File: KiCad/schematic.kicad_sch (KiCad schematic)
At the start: 10 parts, among them J1 AudioJack3, J2 Barrel_Jack_Switch, J3 AudioJack3, SW1 SW_DPDT_x2

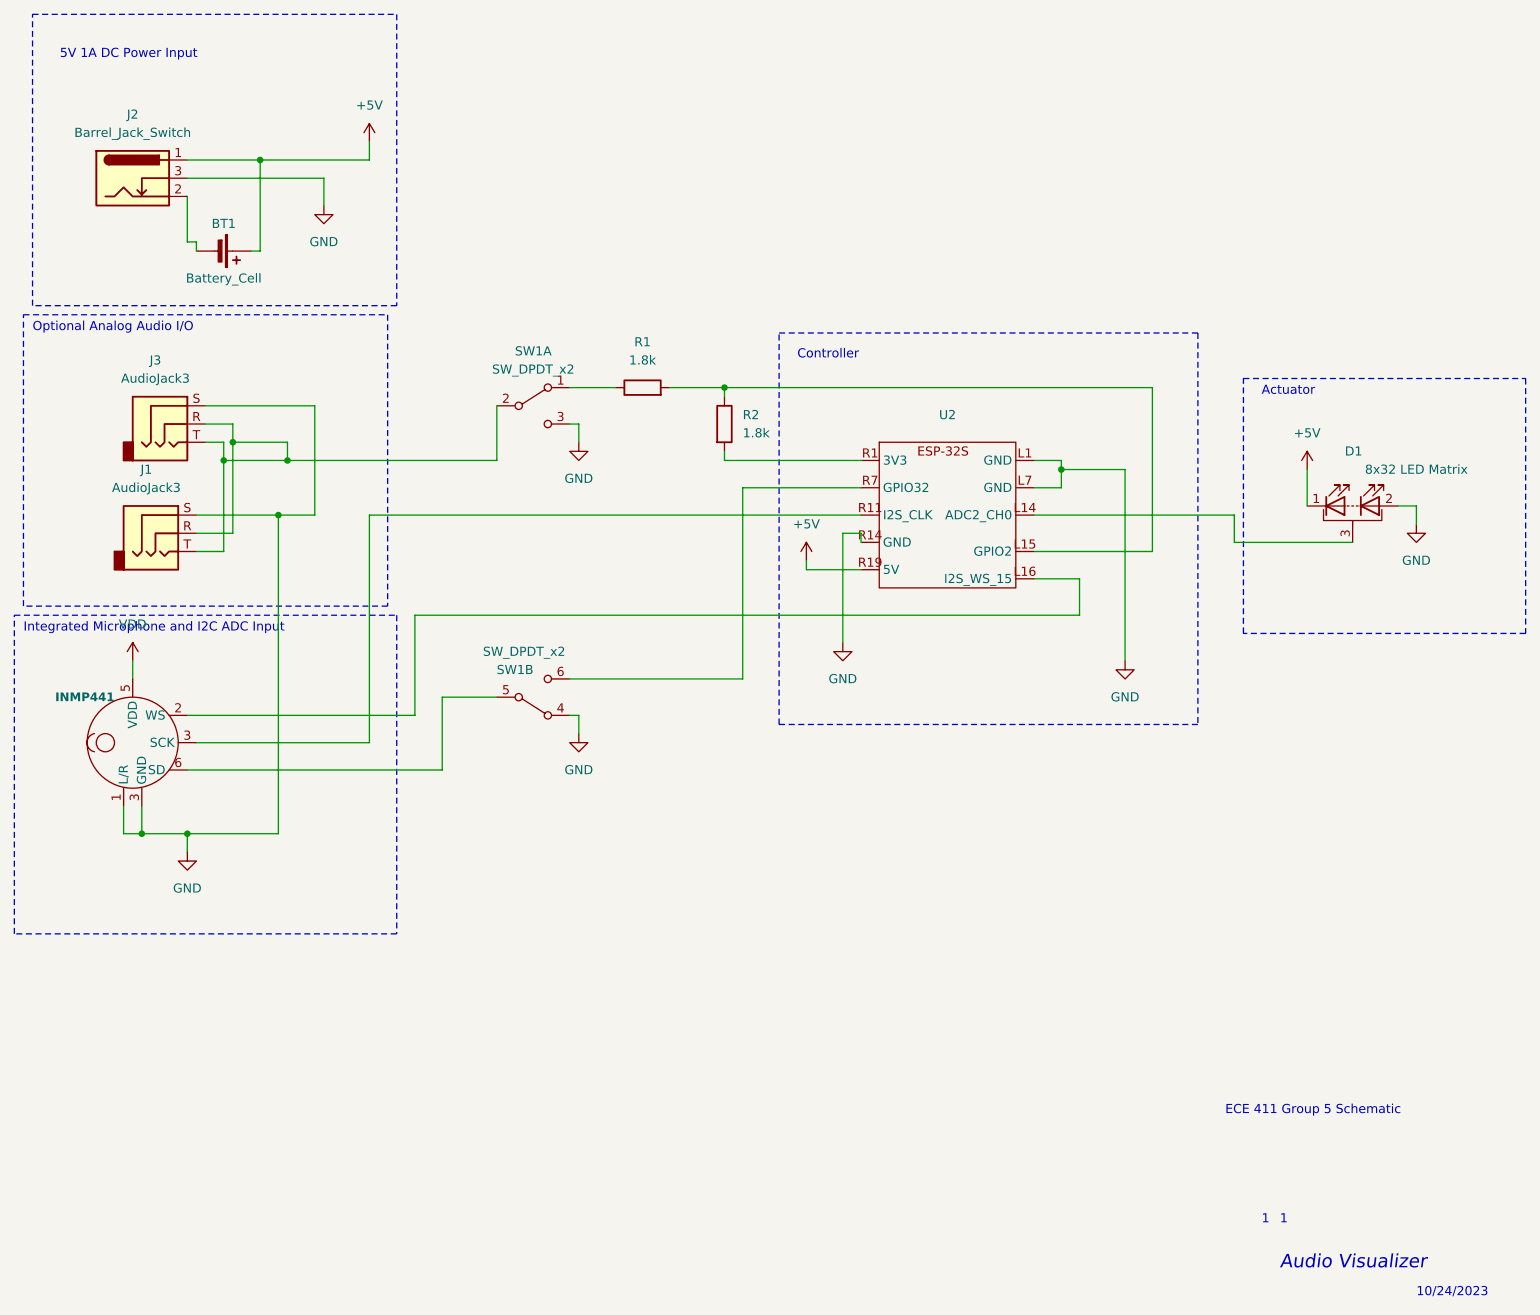
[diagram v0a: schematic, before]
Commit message: update CAD
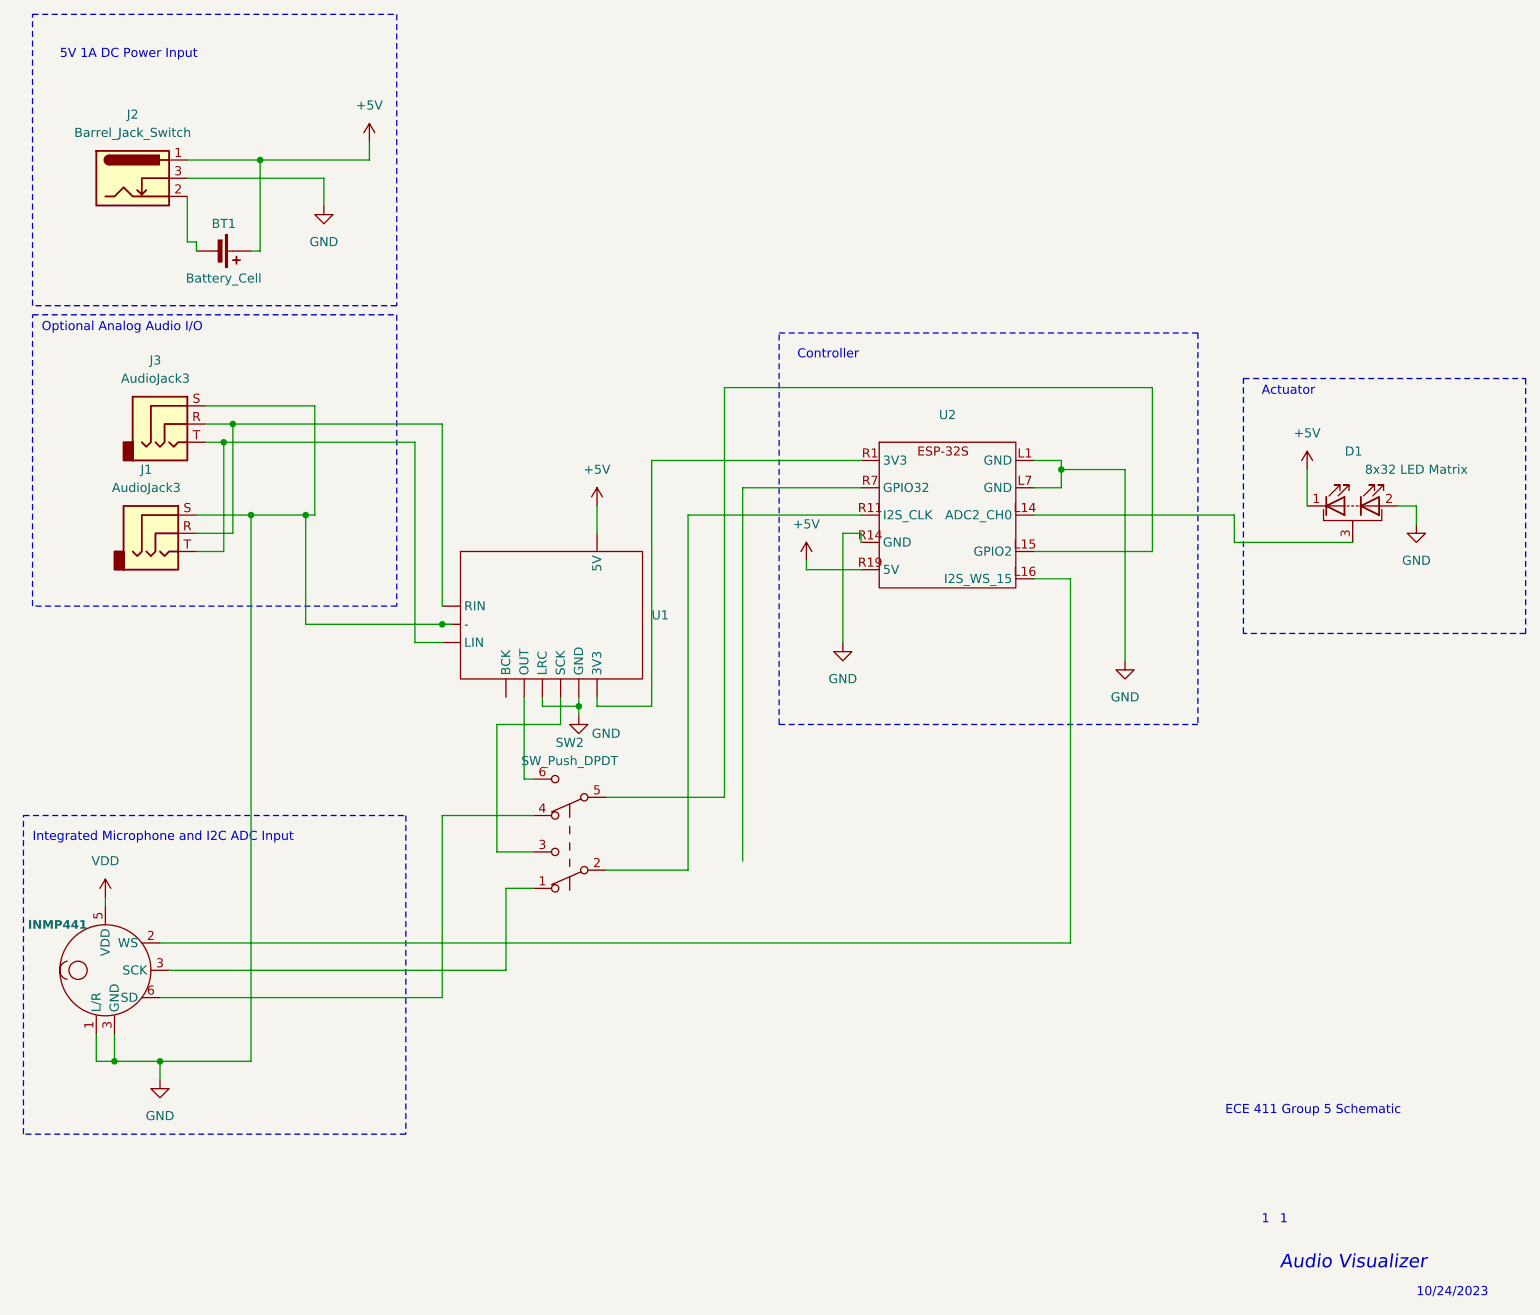
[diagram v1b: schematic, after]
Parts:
- removed R1, R2: 1.8k, symbol Device:R
- removed SW1: SW_DPDT_x2, symbol Switch:SW_DPDT_x2
- added SW2: SW_Push_DPDT, symbol Switch:SW_Push_DPDT
- added U1: ~, symbol MCU_Module:CJMCU-1808
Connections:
- net +5V: now also U1. (SCK)
- net GND: now also U1. (SCK)
- net at J1.R, J3.R: now also U1. (SCK); no longer J1.T, J3.T
- net at U2.L15 (GPIO2): now also SW2.5 (B)
- net at U2.R1 (3V3): now also U1. (SCK)
- net at U2.R11 (I2S_CLK): now also SW2.2 (B); no longer Mic1.3 (SCK)
- net at Mic1.6 (SD): now also SW2.4 (A)
- new net: J1.T, J3.T, U1. (SCK)
- new net: Mic1.3 (SCK), SW2.1 (A)
- new net: SW2.3 (C), U1. (SCK)
- new net: SW2.6 (C), U1. (SCK)
